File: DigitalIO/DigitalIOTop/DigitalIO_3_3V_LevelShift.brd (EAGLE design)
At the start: 66.5 x 62.2 mm, 13 parts, among them K1 HF46105, K2 HF46105, K3 HF46105, K4 HF46105, Q1 691131710002, Q2 691131710002, Q3 691131710002, Q4 691131710002

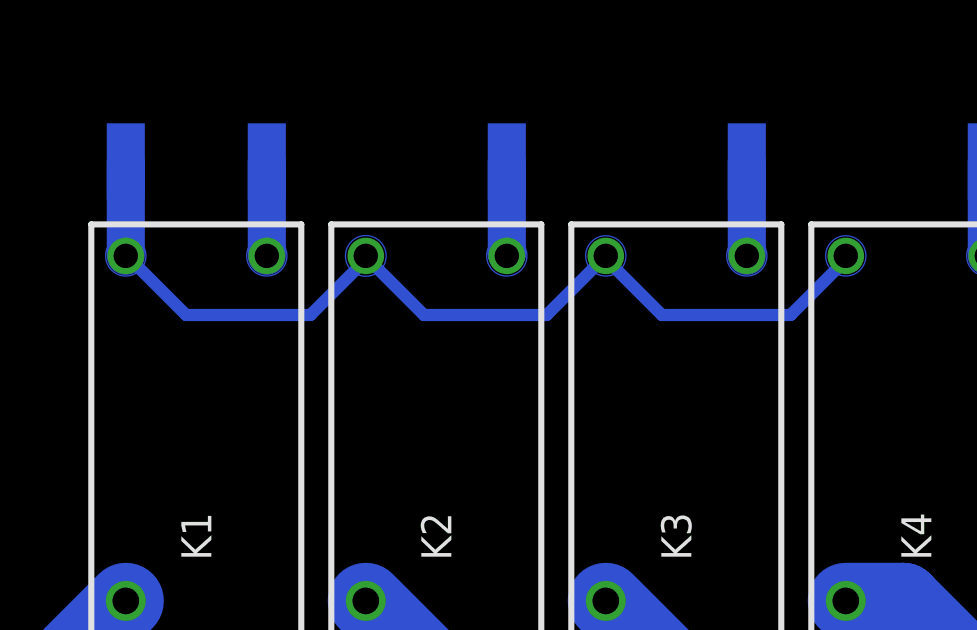
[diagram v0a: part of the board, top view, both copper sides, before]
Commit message: Prepare for production.
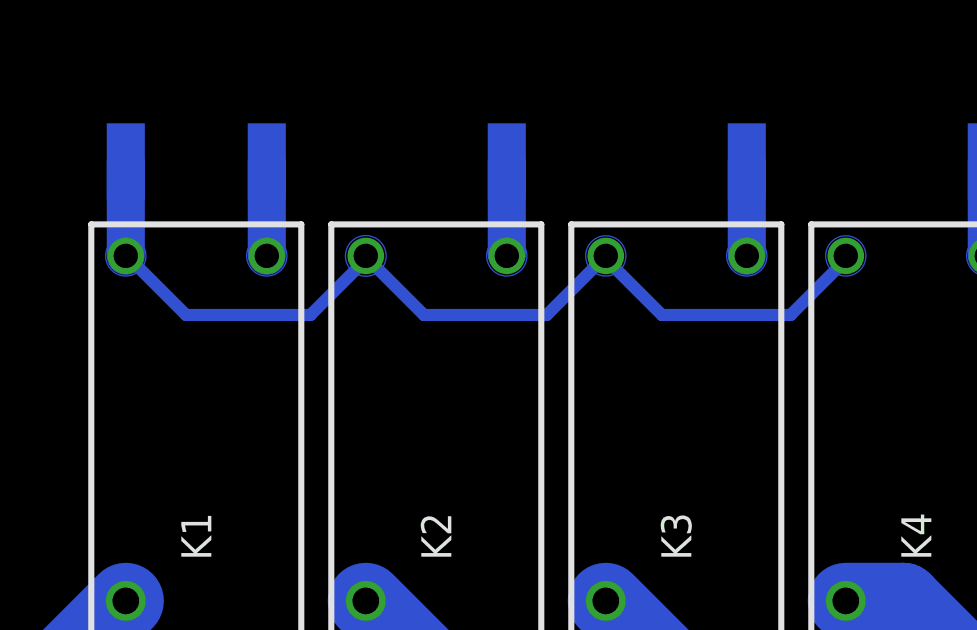
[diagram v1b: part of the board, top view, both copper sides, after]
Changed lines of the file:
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@@
 <wire x1="18.9033" y1="31.925640625" x2="18.9" y2="31.85" width="0.254" layer="16"/>
 <wire x1="28.84" y1="29.88" x2="27.02" y2="31.7" width="0.4064" layer="16"/>
-<wire x1="31.0896" y1="29.88" x2="28.84" y2="29.88" width="0.4064" layer="16"/>
-<wire x1="32.93" y1="29.88" x2="31.0896" y2="29.88" width="0.4064" layer="16"/>
+<wire x1="32.93" y1="29.88" x2="28.84" y2="29.88" width="0.4064" layer="16"/>
 <wire x1="34.75" y1="31.7" x2="32.93" y2="29.88" width="0.4064" layer="16"/>
 <wire x1="27.02" y1="31.7" x2="26.9" y2="31.85" width="0.254" layer="16"/>
 <wire x1="34.75" y1="31.7" x2="34.9" y2="31.85" width="0.254" layer="16"/>
 <wire x1="41.06" y1="29.88" x2="42.88" y2="31.7" width="0.4064" layer="16"/>
-<wire x1="40.03" y1="29.88" x2="41.06" y2="29.88" width="0.4064" layer="16"/>
-<wire x1="36.77" y1="29.88" x2="40.03" y2="29.88" width="0.4064" layer="16"/>
+<wire x1="36.77" y1="29.88" x2="41.06" y2="29.88" width="0.4064" layer="16"/>
 <wire x1="34.95" y1="31.7" x2="36.77" y2="29.88" width="0.4064" layer="16"/>
 <wire x1="42.88" y1="31.7" x2="42.9" y2="31.85" width="0.254" layer="16"/>
 <wire x1="34.95" y1="31.7" x2="34.9" y2="31.85" width="0.254" layer="16"/>
 <wire x1="20.91" y1="29.88" x2="19.1" y2="31.69" width="0.4064" layer="16"/>
-<wire x1="23.070259375" y1="29.88" x2="20.91" y2="29.88" width="0.4064" layer="16"/>
-<wire x1="25.055834375" y1="29.88" x2="23.070259375" y2="29.88" width="0.4064" layer="16"/>
+<wire x1="25.055834375" y1="29.88" x2="20.91" y2="29.88" width="0.4064" layer="16"/>
 <wire x1="26.87585" y1="31.7" x2="25.055834375" y2="29.88" width="0.4064" layer="16"/>
 <wire x1="19.1" y1="31.69" x2="18.9" y2="31.85" width="0.254" layer="16"/>
